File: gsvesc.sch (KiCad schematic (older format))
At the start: 31 parts, among them J1 Conn_01x06, J13 T-Motor, J15 EXT_OFF, J2 Conn_01x06, J3 Conn_01x06, J4 Conn_01x05, J5 Conn_01x03, J6 USB_B_Mini, J7 BAT+, J8 BAT-, U17 TMP100NA_250

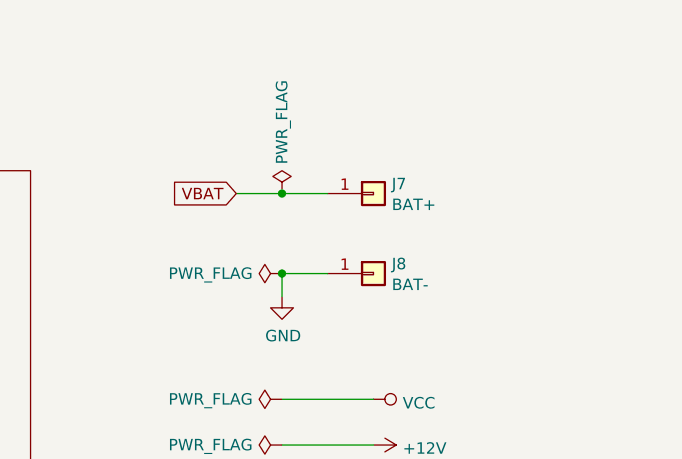
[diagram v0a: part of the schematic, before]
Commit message: temp
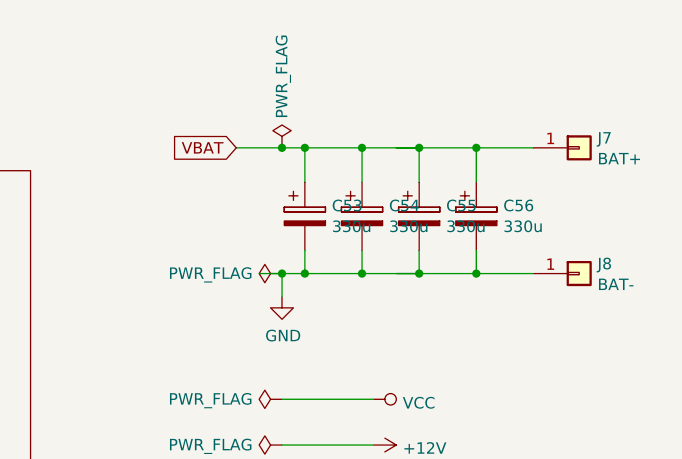
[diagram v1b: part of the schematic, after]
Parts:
- added C53, C54, C55, C56: 330u, Capacitor_SMD:CP_Elec_10x12.5, symbol Device:CP
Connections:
- net GND: now also C53.2, C54.2, C55.2, C56.2
- net VBAT: now also C53.1, C54.1, C55.1, C56.1
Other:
- moved on the sheet: J7, J8
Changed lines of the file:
@@
 L Connector_Generic:Conn_01x01 J7
 U 1 1 5C0450D0
-P 9950 1550
-F 0 "J7" H 10030 1592 50  0000 L CNN
-F 1 "BAT+" H 10030 1501 50  0000 L CNN
-F 2 "gsvesc:TestPoint_Pad_5.0x5.0mm" H 9950 1550 50  0001 C CNN
-F 3 "~" H 9950 1550 50  0001 C CNN
-	1    9950 1550
+P 10850 1350
+F 0 "J7" H 10930 1392 50  0000 L CNN
+F 1 "BAT+" H 10930 1301 50  0000 L CNN
+F 2 "gsvesc:TestPoint_Pad_5.0x5.0mm" H 10850 1350 50  0001 C CNN
+F 3 "~" H 10850 1350 50  0001 C CNN
+	1    10850 1350
 	1    0    0    -1
 $EndComp
@@
 L Connector_Generic:Conn_01x01 J8
 U 1 1 5C045122
-P 9950 1900
-F 0 "J8" H 10030 1942 50  0000 L CNN
-F 1 "BAT-" H 10030 1851 50  0000 L CNN
-F 2 "gsvesc:TestPoint_Pad_5.0x5.0mm" H 9950 1900 50  0001 C CNN
-F 3 "~" H 9950 1900 50  0001 C CNN
-	1    9950 1900
-	1    0    0    -1
-$EndComp
-Wire Wire Line
-	9750 1900 9550 1900
+P 10850 1900
+F 0 "J8" H 10930 1942 50  0000 L CNN
+F 1 "BAT-" H 10930 1851 50  0000 L CNN
+F 2 "gsvesc:TestPoint_Pad_5.0x5.0mm" H 10850 1900 50  0001 C CNN
+F 3 "~" H 10850 1900 50  0001 C CNN
+	1    10850 1900
+	1    0    0    -1
+$EndComp
 $Comp
 L power:GND #PWR019
@@
 L power:PWR_FLAG #FLG0102
 U 1 1 5C34D8D2
-P 9550 1550
-F 0 "#FLG0102" H 9550 1625 50  0001 C CNN
-F 1 "PWR_FLAG" V 9550 1678 50  0000 L CNN
-F 2 "" H 9550 1550 50  0001 C CNN
-F 3 "~" H 9550 1550 50  0001 C CNN
-	1    9550 1550
+P 9550 1350
+F 0 "#FLG0102" H 9550 1425 50  0001 C CNN
+F 1 "PWR_FLAG" V 9550 1478 50  0000 L CNN
+F 2 "" H 9550 1350 50  0001 C CNN
+F 3 "~" H 9550 1350 50  0001 C CNN
+	1    9550 1350
 	1    0    0    -1
 $EndComp
@@
 F15 "CURR_FILTER" I L 7550 3700 50
 $EndSheet
-Wire Wire Line
-	9550 1550 9750 1550
-Text GLabel 9350 1550 0    50   Input ~ 0
+Text GLabel 9350 1350 0    50   Input ~ 0
 VBAT
-Wire Wire Line
-	9550 1550 9350 1550
-Connection ~ 9550 1550
 Wire Wire Line
 	9550 1900 9550 2000
@@
 	0    -1   -1   0
 $EndComp
-Connection ~ 9550 1900
 Wire Wire Line
 	9550 2650 9950 2650
@@
 	8750 5400 8750 5550
 Connection ~ 8750 5550
+Connection ~ 9550 1900
+$Comp
+L Device:CP C53
+U 1 1 5F3842E8
+P 9650 1650
+F 0 "C53" H 9768 1696 50  0000 L CNN
+F 1 "330u" H 9768 1605 50  0000 L CNN
+F 2 "Capacitor_SMD:CP_Elec_10x12.5" H 9688 1500 50  0001 C CNN
+F 3 "~" H 9650 1650 50  0001 C CNN
+	1    9650 1650
+	1    0    0    -1
+$EndComp
+$Comp
+L Device:CP C54
+U 1 1 5F3843DA
+P 9900 1650
+F 0 "C54" H 10018 1696 50  0000 L CNN
+F 1 "330u" H 10018 1605 50  0000 L CNN
+F 2 "Capacitor_SMD:CP_Elec_10x12.5" H 9938 1500 50  0001 C CNN
+F 3 "~" H 9900 1650 50  0001 C CNN
+	1    9900 1650
+	1    0    0    -1
+$EndComp
+Wire Wire Line
+	9650 1500 9650 1350
+Connection ~ 9650 1350
+Wire Wire Line
+	9650 1350 9900 1350
+Wire Wire Line
+	9650 1800 9650 1900
+Connection ~ 9650 1900
+Wire Wire Line
+	9650 1900 9550 1900
+Wire Wire Line
+	9900 1800 9900 1900
+Wire Wire Line
+	9900 1500 9900 1350
+Wire Wire Line
+	9550 1350 9650 1350
+Wire Wire Line
+	9550 1900 9450 1900
+Wire Wire Line
+	9350 1350 9550 1350
+Connection ~ 9900 1350
+Connection ~ 9900 1900
+Wire Wire Line
+	9900 1900 9650 1900
+Connection ~ 9550 1350
+$Comp
+L Device:CP C55
+U 1 1 5F3B3A44
+P 10150 1650
+F 0 "C55" H 10268 1696 50  0000 L CNN
+F 1 "330u" H 10268 1605 50  0000 L CNN
+F 2 "Capacitor_SMD:CP_Elec_10x12.5" H 10188 1500 50  0001 C CNN
+F 3 "~" H 10150 1650 50  0001 C CNN
+	1    10150 1650
+	1    0    0    -1
+$EndComp
+$Comp
+L Device:CP C56
+U 1 1 5F3B3A4A
+P 10400 1650
+F 0 "C56" H 10518 1696 50  0000 L CNN
+F 1 "330u" H 10518 1605 50  0000 L CNN
+F 2 "Capacitor_SMD:CP_Elec_10x12.5" H 10438 1500 50  0001 C CNN
+F 3 "~" H 10400 1650 50  0001 C CNN
+	1    10400 1650
+	1    0    0    -1
+$EndComp
+Wire Wire Line
+	10150 1500 10150 1350
+Connection ~ 10150 1350
+Wire Wire Line
+	10150 1350 10400 1350
+Wire Wire Line
+	10150 1800 10150 1900
+Connection ~ 10150 1900
+Wire Wire Line
+	10400 1800 10400 1900
+Wire Wire Line
+	10400 1500 10400 1350
+Connection ~ 10400 1350
+Connection ~ 10400 1900
+Wire Wire Line
+	10400 1900 10150 1900
+Wire Wire Line
+	10400 1350 10650 1350
+Wire Wire Line
+	10400 1900 10650 1900
+Wire Wire Line
+	10050 1350 10150 1350
+Wire Wire Line
+	10050 1900 10150 1900
+Wire Wire Line
+	9900 1350 10150 1350
+Wire Wire Line
+	9900 1900 10150 1900
 $EndSCHEMATC
